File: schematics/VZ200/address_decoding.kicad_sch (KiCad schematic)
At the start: 43 parts, among them J901 Cassette, J903 Keyboard, Q900 9018, U1 74LS174, U12 74LS244, U2 74LS32, U3 74LS139

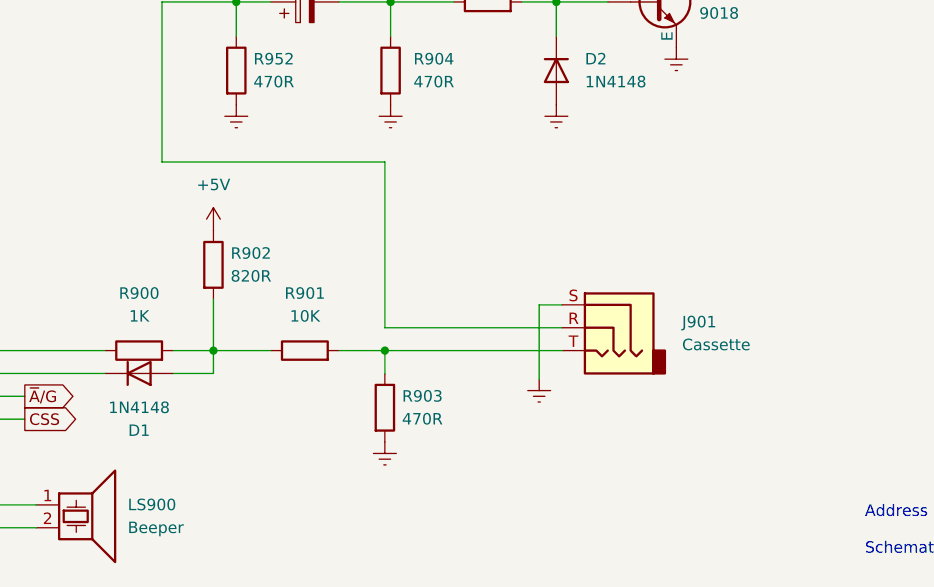
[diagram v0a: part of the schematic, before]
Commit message: Restoration Part 2
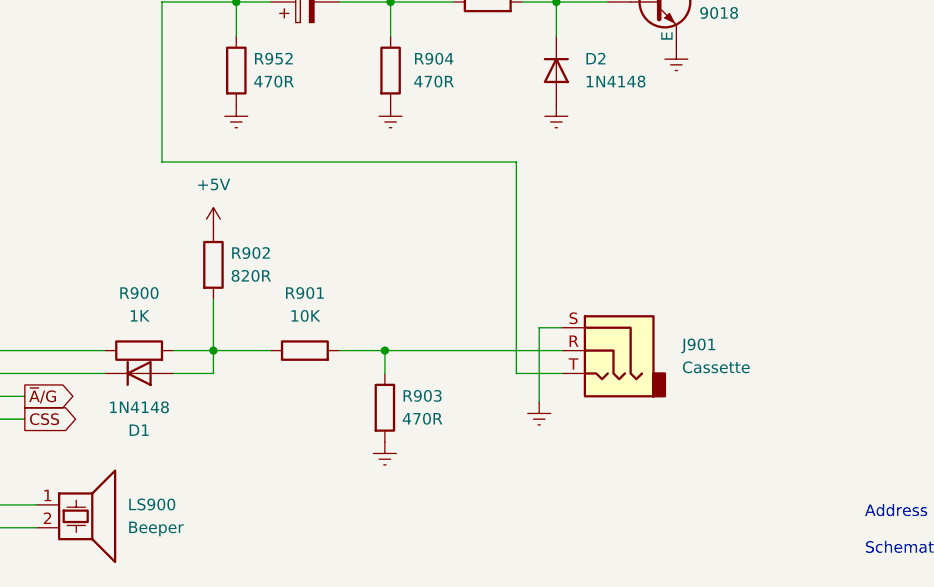
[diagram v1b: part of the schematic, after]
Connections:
- net at C905.1, R952.1: now also J901.T; no longer J901.R
- net at R901.2, R903.1: now also J901.R; no longer J901.T
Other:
- moved on the sheet: J901
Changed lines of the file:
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@@
   (junction (at 112.395 50.165) (diameter 0) (color 0 0 0 0)
   )
+  (junction (at 128.905 153.67) (diameter 0) (color 0 0 0 0)
+  )
   (junction (at 178.435 71.755) (diameter 0) (color 0 0 0 0)
   )
@@
   (junction (at 198.755 84.455) (diameter 0) (color 0 0 0 0)
   )
-  (junction (at 128.905 153.67) (diameter 0) (color 0 0 0 0)
-  )
   (junction (at 112.395 114.935) (diameter 0) (color 0 0 0 0)
   )
@@
     (stroke (width 0) (type default))
   )
-  (wire (pts (xy 148.59 148.59) (xy 146.05 148.59))
-    (stroke (width 0) (type default))
-  )
   (bus (pts (xy 228.6 153.035) (xy 231.14 153.035))
     (stroke (width 0) (type default))
@@
     (stroke (width 0) (type default))
   )
-  (wire (pts (xy 148.59 151.13) (xy 128.905 151.13))
+  (wire (pts (xy 104.14 132.715) (xy 104.14 114.935))
     (stroke (width 0) (type default))
   )
-  (wire (pts (xy 104.14 132.715) (xy 104.14 114.935))
+  (wire (pts (xy 148.59 156.21) (xy 143.51 156.21))
     (stroke (width 0) (type default))
   )
@@
     (stroke (width 0) (type default))
   )
+  (wire (pts (xy 128.905 153.67) (xy 148.59 153.67))
+    (stroke (width 0) (type default))
+  )
   (bus (pts (xy 278.13 88.265) (xy 278.13 85.09))
     (stroke (width 0) (type default))
@@
     (stroke (width 0) (type default))
   )
-  (wire (pts (xy 146.05 148.59) (xy 146.05 156.845))
-    (stroke (width 0) (type default))
-  )
-  (wire (pts (xy 128.905 153.67) (xy 148.59 153.67))
+  (wire (pts (xy 146.05 151.13) (xy 146.05 159.385))
     (stroke (width 0) (type default))
   )
@@
     (stroke (width 0) (type default))
   )
+  (wire (pts (xy 146.05 151.13) (xy 148.59 151.13))
+    (stroke (width 0) (type default))
+  )
   (wire (pts (xy 116.205 53.34) (xy 149.86 53.34))
     (stroke (width 0) (type default))
@@
     (stroke (width 0) (type default))
   )
-  (wire (pts (xy 128.905 151.13) (xy 128.905 132.715))
+  (wire (pts (xy 143.51 132.715) (xy 143.51 156.21))
     (stroke (width 0) (type default))
   )
@@
     (stroke (width 0) (type default))
   )
-  (wire (pts (xy 128.905 132.715) (xy 104.14 132.715))
+  (wire (pts (xy 143.51 132.715) (xy 104.14 132.715))
     (stroke (width 0) (type default))
   )
@@
     )
   )
-  (symbol (lib_id "power:Earth") (at 146.05 156.845 0) (unit 1)
+  (symbol (lib_id "power:Earth") (at 146.05 159.385 0) (unit 1)
     (in_bom yes) (on_board yes) (dnp no) (fields_autoplaced)
-    (property "Reference" "#PWR039" (at 146.05 163.195 0)
+    (property "Reference" "#PWR039" (at 146.05 165.735 0)
       (effects (font (size 1.27 1.27)) hide)
     )
-    (property "Value" "Earth" (at 146.05 160.655 0)
+    (property "Value" "Earth" (at 146.05 163.195 0)
       (effects (font (size 1.27 1.27)) hide)
     )
-    (property "Footprint" "" (at 146.05 156.845 0)
+    (property "Footprint" "" (at 146.05 159.385 0)
       (effects (font (size 1.27 1.27)) hide)
     )
-    (property "Datasheet" "~" (at 146.05 156.845 0)
+    (property "Datasheet" "~" (at 146.05 159.385 0)
       (effects (font (size 1.27 1.27)) hide)
     )
@@
     )
   )
-  (symbol (lib_id "Connector_Audio:AudioJack3") (at 153.67 151.13 0) (mirror y) (unit 1)
+  (symbol (lib_id "Connector_Audio:AudioJack3") (at 153.67 153.67 0) (mirror y) (unit 1)
     (in_bom yes) (on_board yes) (dnp no) (fields_autoplaced)
-    (property "Reference" "J901" (at 161.925 150.495 0)
+    (property "Reference" "J901" (at 161.925 153.035 0)
       (effects (font (size 1.27 1.27)) (justify right))
     )
-    (property "Value" "Cassette" (at 161.925 153.035 0)
+    (property "Value" "Cassette" (at 161.925 155.575 0)
       (effects (font (size 1.27 1.27)) (justify right))
     )
-    (property "Footprint" "" (at 153.67 151.13 0)
+    (property "Footprint" "" (at 153.67 153.67 0)
       (effects (font (size 1.27 1.27)) hide)
     )
-    (property "Datasheet" "~" (at 153.67 151.13 0)
+    (property "Datasheet" "~" (at 153.67 153.67 0)
       (effects (font (size 1.27 1.27)) hide)
     )
